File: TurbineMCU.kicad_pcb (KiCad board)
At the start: 4 copper layers, 53.7 x 54.7 mm, 45 parts, among them IC1 MSPM0G3507SPMR, IC2 TPS73533DRVT, J1 Conn_01x02_Socket, J10 Conn_01x03_Socket, J13 Conn_01x03_Socket, J14 Conn_01x03_Socket, J15 Conn_01x08_Pin, J2 Conn_01x02_Socket, J3 Conn_01x04_Socket, J5 Conn_01x03_Socket, J6 Conn_01x03_Socket, J8 Conn_01x03_Socket, SW1 SW_Push, SW2 SW_Push

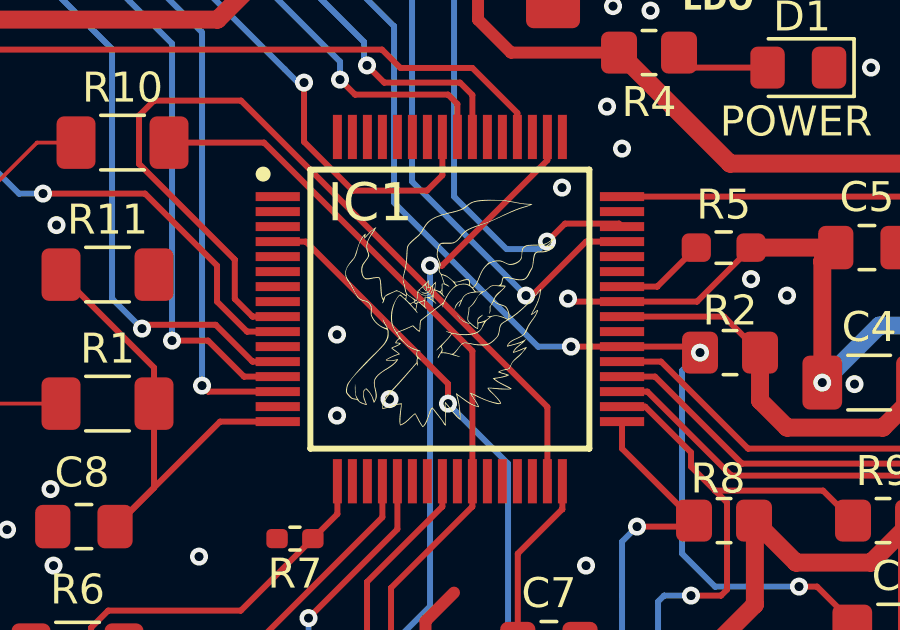
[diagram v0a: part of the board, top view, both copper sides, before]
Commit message: board finished
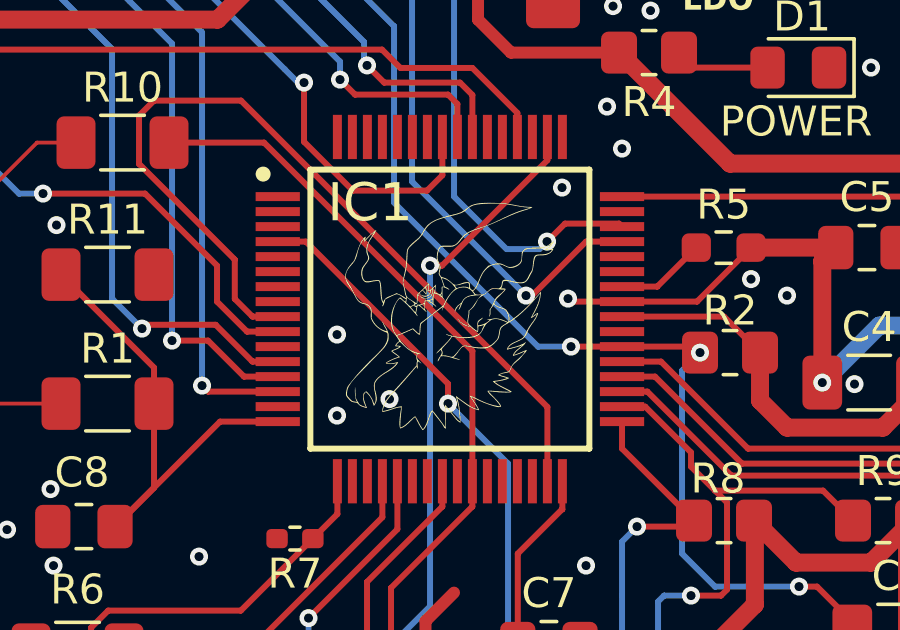
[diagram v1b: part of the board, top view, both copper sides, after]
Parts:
- moved G*** 0.10 mm to (171.3, 92.1)
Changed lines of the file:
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@@
 	(footprint "LOGO"
 		(layer "F.Cu")
-		(at 171.262 92)
+		(at 171.262 92.1)
 		(property "Reference" "G***"
 			(at 0 0 0)
